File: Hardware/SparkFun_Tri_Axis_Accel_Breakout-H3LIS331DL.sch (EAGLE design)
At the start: 23 parts, among them U1 H3LIS331DL

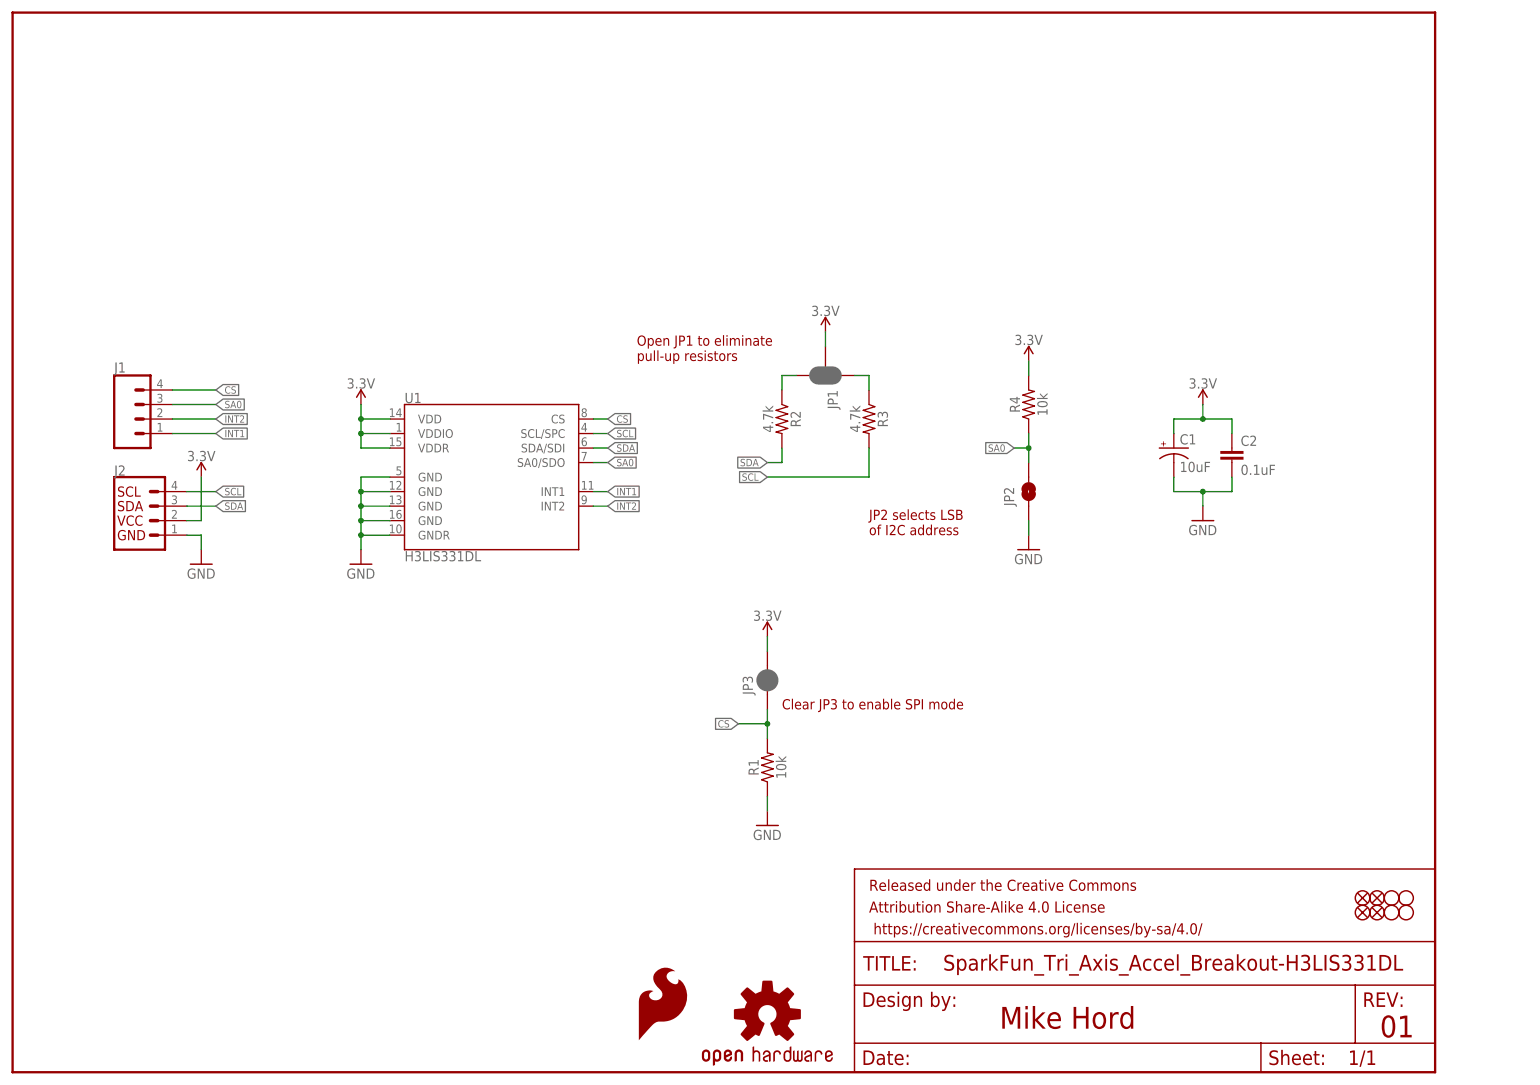
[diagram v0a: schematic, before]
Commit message: Aesthetic touch ups before review
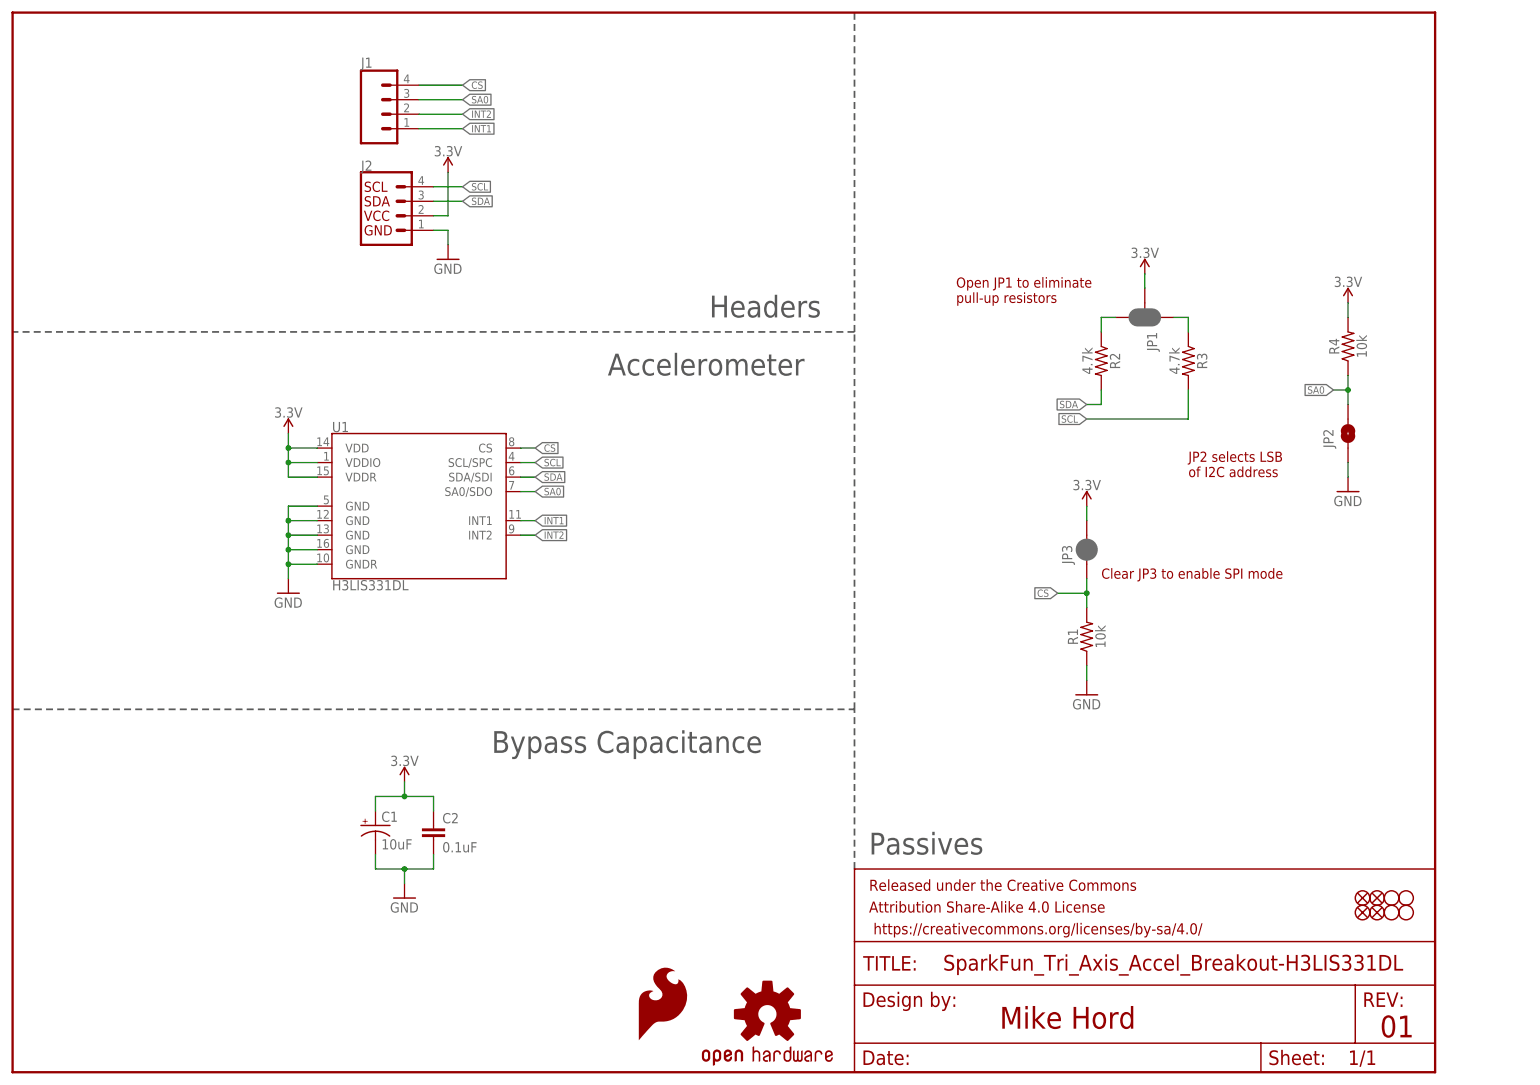
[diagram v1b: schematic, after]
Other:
- note added: "Accelerometer"
- note added: "Bypass Capacitance"
- note added: "Headers"
- note added: "Passives"
- moved on the sheet: C1, C2, J1, J2, JP1, JP2, JP3, R1, R2, R3, R4, U1

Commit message: Replace some components with newer versions
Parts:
- C1: device SparkFun:CAP_POL1206 -> SparkFun-Capacitors:10UF-POLAR-EIA3216-16V-10%(TANT)
- C2: device SparkFun:CAP0402-CAP -> SparkFun-Capacitors:0.1UF-0603-25V-5%
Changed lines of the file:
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@@
 </classes>
 <parts>
-<part name="C2" library="SparkFun" deviceset="CAP" device="0402-CAP" value="0.1uF"/>
+<part name="C2" library="SparkFun-Capacitors" deviceset="0.1UF" device="-0603-25V-5%" value="0.1uF"/>
 <part name="GND1" library="SparkFun" deviceset="GND" device=""/>
 <part name="GND5" library="SparkFun" deviceset="GND" device=""/>
 <part name="U1" library="SparkFun-Sensors" deviceset="H3LIS331DL" device="" value="H3LIS331DL"/>
 <part name="GND2" library="SparkFun" deviceset="GND" device=""/>
-<part name="C1" library="SparkFun" deviceset="CAP_POL" device="1206" value="10uF"/>
+<part name="C1" library="SparkFun-Capacitors" deviceset="10UF-POLAR" device="-EIA3216-16V-10%(TANT)" value="10uF"/>
 <part name="JP11" library="SparkFun" deviceset="STAND-OFF" device=""/>
 <part name="JP10" library="SparkFun" deviceset="STAND-OFF" device=""/>
